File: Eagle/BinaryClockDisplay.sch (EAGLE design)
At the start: 45 parts

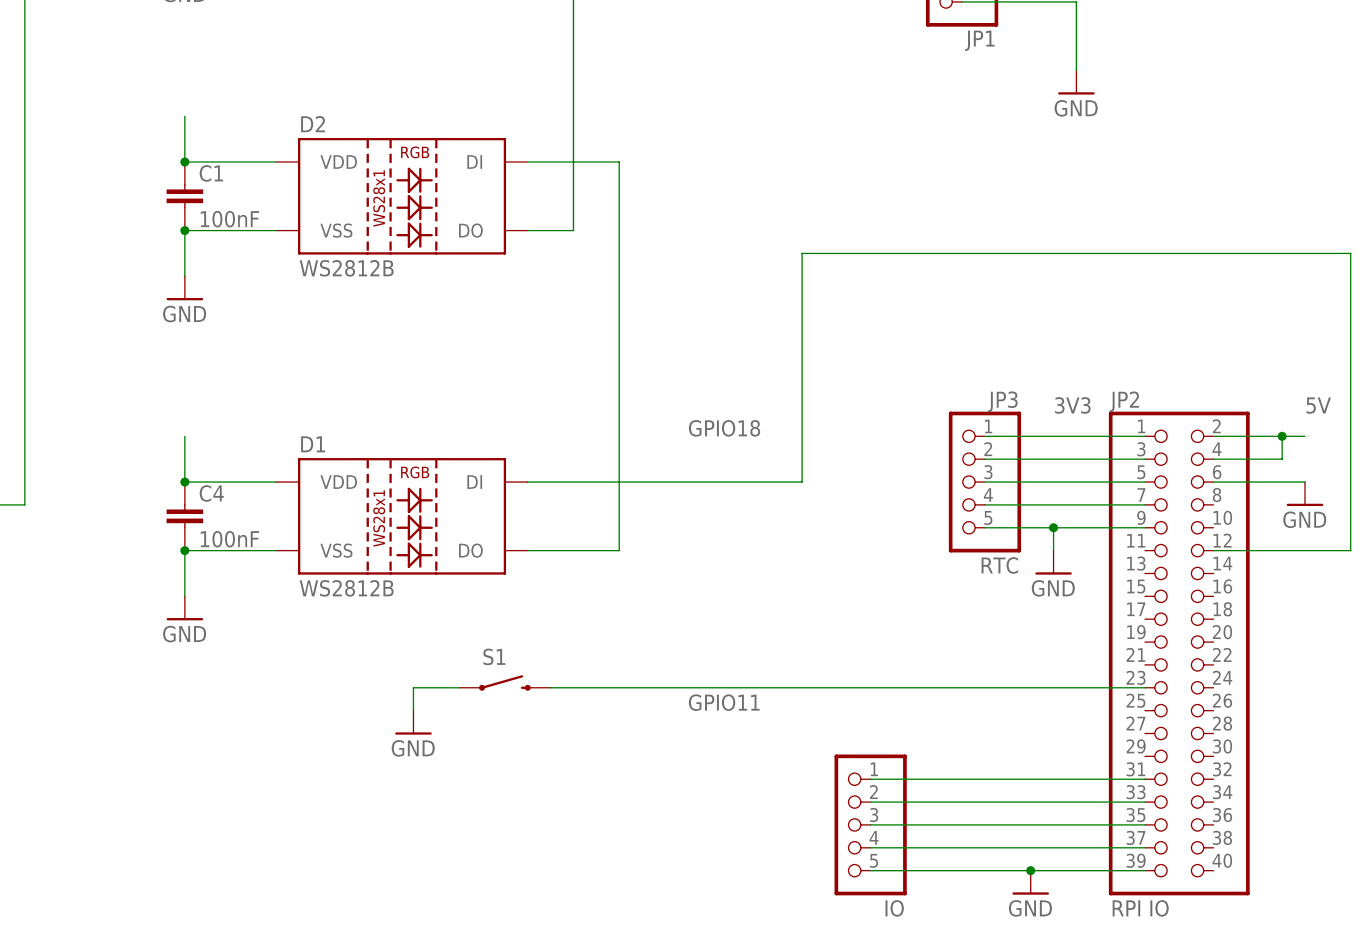
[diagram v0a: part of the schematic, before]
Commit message: HW version 2 allmost done...
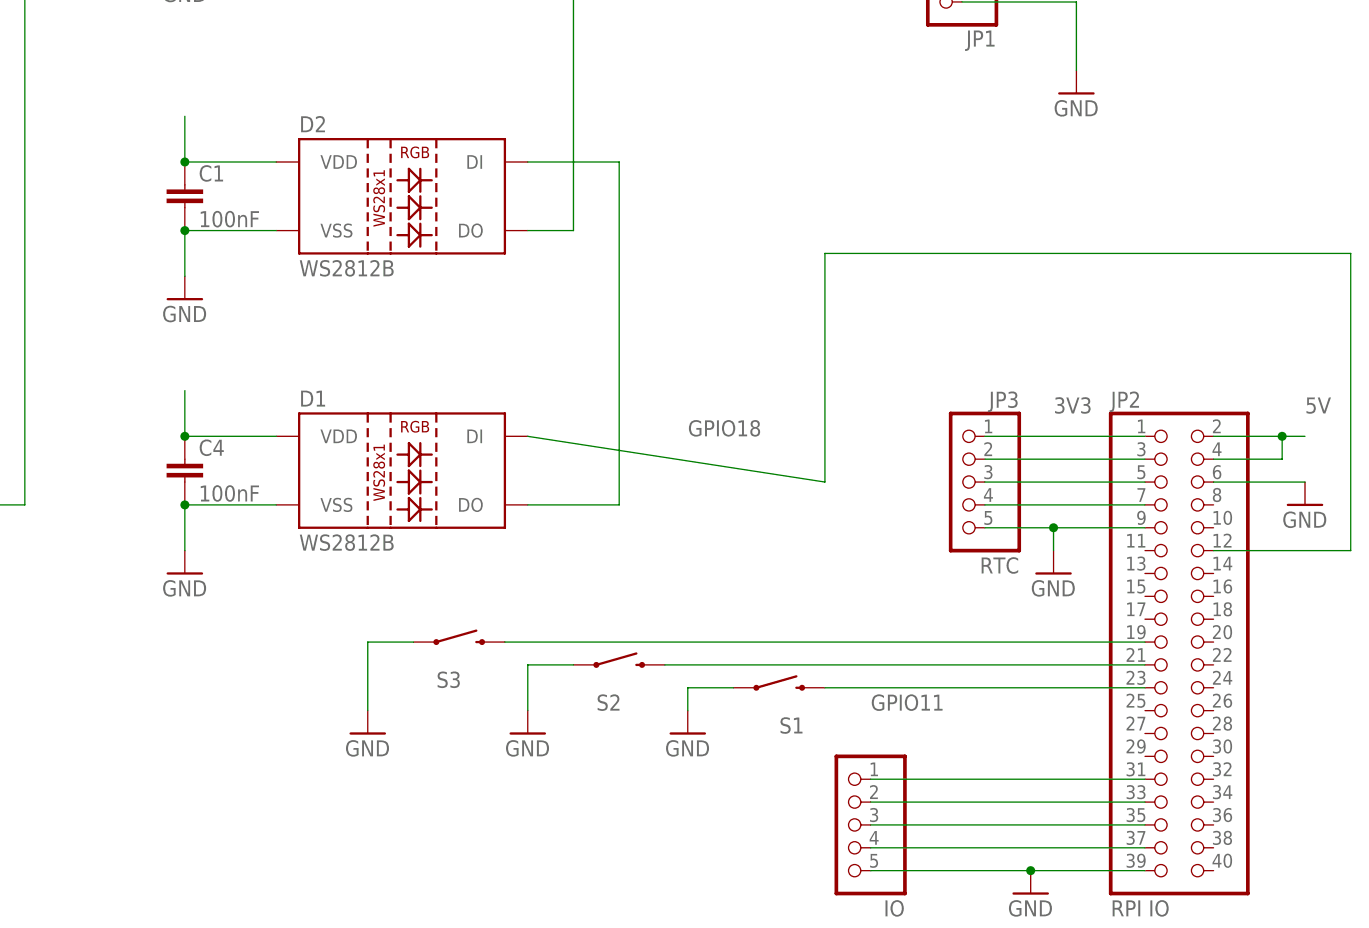
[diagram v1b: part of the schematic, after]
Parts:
- added S2, S3: SWITCH, SparkFun-Electromechanical:SWITCH-MOMENTARY-2SMD-1101NE
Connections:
- new net GPIO10: JP2.19, S3.2
- new net GPIO9: JP2.21, S2.2
- net GND: now also S2.1, S3.1
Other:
- moved on the sheet: C4, D1, S1
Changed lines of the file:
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@@
 <part name="GND25" library="supply1" deviceset="GND" device=""/>
 <part name="JP4" library="pinhead" library_urn="urn:adsk.eagle:library:325" deviceset="PINHD-1X5" device="" package3d_urn="urn:adsk.eagle:package:22469/2" value="IO"/>
+<part name="S2" library="SparkFun-Electromechanical" deviceset="SWITCH-MOMENTARY-2" device="SMD-1101NE" value="SWITCH"/>
+<part name="GND26" library="supply1" deviceset="GND" device=""/>
+<part name="S3" library="SparkFun-Electromechanical" deviceset="SWITCH-MOMENTARY-2" device="SMD-1101NE" value="SWITCH"/>
+<part name="GND27" library="supply1" deviceset="GND" device=""/>
 </parts>
 <sheets>
@@
 </plain>
 <instances>
-<instance part="D1" gate="G$1" x="129.54" y="35.56" smashed="yes">
-<attribute name="NAME" x="116.84" y="43.942" size="1.778" layer="95"/>
-<attribute name="VALUE" x="116.84" y="27.94" size="1.778" layer="95"/>
+<instance part="D1" gate="G$1" x="129.54" y="40.64" smashed="yes">
+<attribute name="NAME" x="116.84" y="49.022" size="1.778" layer="95"/>
+<attribute name="VALUE" x="116.84" y="33.02" size="1.778" layer="95"/>
 </instance>
 <instance part="JP2" gate="A" x="213.36" y="22.86" smashed="yes">
@@
 <attribute name="VALUE" x="207.01" y="-7.62" size="1.778" layer="96"/>
 </instance>
-<instance part="C4" gate="G$1" x="104.14" y="35.56" smashed="yes">
-<attribute name="NAME" x="105.664" y="38.481" size="1.778" layer="95"/>
-<attribute name="VALUE" x="105.664" y="33.401" size="1.778" layer="96"/>
+<instance part="C4" gate="G$1" x="104.14" y="40.64" smashed="yes">
+<attribute name="NAME" x="105.664" y="43.561" size="1.778" layer="95"/>
+<attribute name="VALUE" x="105.664" y="38.481" size="1.778" layer="96"/>
 </instance>
 <instance part="JP3" gate="A" x="190.5" y="40.64" smashed="yes" rot="MR0">
@@
 <attribute name="VALUE" x="196.85" y="30.48" size="1.778" layer="96" rot="MR0"/>
 </instance>
-<instance part="GND10" gate="1" x="104.14" y="25.4" smashed="yes">
-<attribute name="VALUE" x="101.6" y="22.86" size="1.778" layer="96"/>
+<instance part="GND10" gate="1" x="104.14" y="30.48" smashed="yes">
+<attribute name="VALUE" x="101.6" y="27.94" size="1.778" layer="96"/>
 </instance>
 <instance part="D2" gate="G$1" x="129.54" y="71.12" smashed="yes">
@@
 <attribute name="VALUE" x="-238.76" y="43.18" size="1.778" layer="96"/>
 </instance>
-<instance part="S1" gate="G$1" x="139.7" y="17.78" smashed="yes">
-<attribute name="NAME" x="137.16" y="20.32" size="1.778" layer="95"/>
-</instance>
-<instance part="GND22" gate="1" x="129.54" y="12.7" smashed="yes">
-<attribute name="VALUE" x="127" y="10.16" size="1.778" layer="96"/>
+<instance part="S1" gate="G$1" x="170.18" y="17.78" smashed="yes">
+<attribute name="NAME" x="170.18" y="12.7" size="1.778" layer="95"/>
+</instance>
+<instance part="GND22" gate="1" x="160.02" y="12.7" smashed="yes">
+<attribute name="VALUE" x="157.48" y="10.16" size="1.778" layer="96"/>
 </instance>
 <instance part="GND23" gate="1" x="198.12" y="-5.08" smashed="yes">
@@
 <instance part="JP4" gate="A" x="177.8" y="2.54" smashed="yes" rot="MR0">
 <attribute name="VALUE" x="184.15" y="-7.62" size="1.778" layer="96" rot="MR0"/>
+</instance>
+<instance part="S2" gate="G$1" x="152.4" y="20.32" smashed="yes">
+<attribute name="NAME" x="149.86" y="15.24" size="1.778" layer="95"/>
+</instance>
+<instance part="GND26" gate="1" x="142.24" y="12.7" smashed="yes">
+<attribute name="VALUE" x="139.7" y="10.16" size="1.778" layer="96"/>
+</instance>
+<instance part="S3" gate="G$1" x="134.62" y="22.86" smashed="yes">
+<attribute name="NAME" x="132.08" y="17.78" size="1.778" layer="95"/>
+</instance>
+<instance part="GND27" gate="1" x="124.46" y="12.7" smashed="yes">
+<attribute name="VALUE" x="121.92" y="10.16" size="1.778" layer="96"/>
 </instance>
 </instances>
@@
 <pinref part="D1" gate="G$1" pin="VSS"/>
 <pinref part="C4" gate="G$1" pin="2"/>
-<wire x1="114.3" y1="33.02" x2="104.14" y2="33.02" width="0.1524" layer="91"/>
-<wire x1="104.14" y1="33.02" x2="104.14" y2="27.94" width="0.1524" layer="91"/>
-<junction x="104.14" y="33.02"/>
+<wire x1="114.3" y1="38.1" x2="104.14" y2="38.1" width="0.1524" layer="91"/>
+<wire x1="104.14" y1="38.1" x2="104.14" y2="33.02" width="0.1524" layer="91"/>
+<junction x="104.14" y="38.1"/>
 <pinref part="GND10" gate="1" pin="GND"/>
 </segment>
@@
 <pinref part="S1" gate="G$1" pin="1"/>
 <pinref part="GND22" gate="1" pin="GND"/>
-<wire x1="134.62" y1="17.78" x2="129.54" y2="17.78" width="0.1524" layer="91"/>
-<wire x1="129.54" y1="17.78" x2="129.54" y2="15.24" width="0.1524" layer="91"/>
+<wire x1="165.1" y1="17.78" x2="160.02" y2="17.78" width="0.1524" layer="91"/>
+<wire x1="160.02" y1="17.78" x2="160.02" y2="15.24" width="0.1524" layer="91"/>
 </segment>
 <segment>
@@
 <pinref part="GND25" gate="1" pin="GND"/>
 </segment>
+<segment>
+<pinref part="S2" gate="G$1" pin="1"/>
+<pinref part="GND26" gate="1" pin="GND"/>
+<wire x1="147.32" y1="20.32" x2="142.24" y2="20.32" width="0.1524" layer="91"/>
+<wire x1="142.24" y1="20.32" x2="142.24" y2="15.24" width="0.1524" layer="91"/>
+</segment>
+<segment>
+<pinref part="S3" gate="G$1" pin="1"/>
+<pinref part="GND27" gate="1" pin="GND"/>
+<wire x1="129.54" y1="22.86" x2="124.46" y2="22.86" width="0.1524" layer="91"/>
+<wire x1="124.46" y1="22.86" x2="124.46" y2="15.24" width="0.1524" layer="91"/>
+</segment>
 </net>
 <net name="N$2" class="0">
@@
 <segment>
 <pinref part="D1" gate="G$1" pin="DO"/>
-<wire x1="142.24" y1="33.02" x2="152.4" y2="33.02" width="0.1524" layer="91"/>
+<wire x1="142.24" y1="38.1" x2="152.4" y2="38.1" width="0.1524" layer="91"/>
 <pinref part="D2" gate="G$1" pin="DI"/>
-<wire x1="152.4" y1="33.02" x2="152.4" y2="76.2" width="0.1524" layer="91"/>
+<wire x1="152.4" y1="38.1" x2="152.4" y2="76.2" width="0.1524" layer="91"/>
 <wire x1="152.4" y1="76.2" x2="142.24" y2="76.2" width="0.1524" layer="91"/>
 </segment>
@@
 <segment>
 <pinref part="D1" gate="G$1" pin="DI"/>
-<wire x1="172.72" y1="40.64" x2="142.24" y2="40.64" width="0.1524" layer="91"/>
-<wire x1="233.68" y1="66.04" x2="172.72" y2="66.04" width="0.1524" layer="91"/>
-<wire x1="172.72" y1="66.04" x2="172.72" y2="40.64" width="0.1524" layer="91"/>
+<wire x1="175.26" y1="40.64" x2="142.24" y2="45.72" width="0.1524" layer="91"/>
+<wire x1="233.68" y1="66.04" x2="175.26" y2="66.04" width="0.1524" layer="91"/>
+<wire x1="175.26" y1="66.04" x2="175.26" y2="40.64" width="0.1524" layer="91"/>
 <label x="160.02" y="45.72" size="1.778" layer="95"/>
 <wire x1="233.68" y1="66.04" x2="233.68" y2="33.02" width="0.1524" layer="91"/>
@@
 <pinref part="S1" gate="G$1" pin="2"/>
 <pinref part="JP2" gate="A" pin="23"/>
-<wire x1="144.78" y1="17.78" x2="210.82" y2="17.78" width="0.1524" layer="91"/>
-<label x="160.02" y="15.24" size="1.778" layer="95"/>
+<wire x1="175.26" y1="17.78" x2="210.82" y2="17.78" width="0.1524" layer="91"/>
+<label x="180.34" y="15.24" size="1.778" layer="95"/>
 </segment>
 </net>
@@
 <pinref part="C4" gate="G$1" pin="1"/>
 <pinref part="D1" gate="G$1" pin="VDD"/>
-<wire x1="104.14" y1="40.64" x2="114.3" y2="40.64" width="0.1524" layer="91"/>
-<wire x1="104.14" y1="40.64" x2="104.14" y2="45.72" width="0.1524" layer="91"/>
-<junction x="104.14" y="40.64"/>
+<wire x1="104.14" y1="45.72" x2="114.3" y2="45.72" width="0.1524" layer="91"/>
+<wire x1="104.14" y1="45.72" x2="104.14" y2="50.8" width="0.1524" layer="91"/>
+<junction x="104.14" y="45.72"/>
 </segment>
 <segment>
@@
 </segment>
 </net>
+<net name="GPIO9" class="0">
+<segment>
+<pinref part="S2" gate="G$1" pin="2"/>
+<wire x1="157.48" y1="20.32" x2="210.82" y2="20.32" width="0.1524" layer="91"/>
+<pinref part="JP2" gate="A" pin="21"/>
+</segment>
+</net>
+<net name="GPIO10" class="0">
+<segment>
+<pinref part="S3" gate="G$1" pin="2"/>
+<pinref part="JP2" gate="A" pin="19"/>
+<wire x1="139.7" y1="22.86" x2="210.82" y2="22.86" width="0.1524" layer="91"/>
+</segment>
+</net>
